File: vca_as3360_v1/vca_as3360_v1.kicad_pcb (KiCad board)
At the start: 2 copper layers, 30 x 100 mm, 71 parts, among them J1 Conn_02x05_Odd_Even, J2 OUT_1, J3 OUT_2, J4 CV1, J5 CV2, J6 IN1, J7 IN2, Q1 BC547, Q2 BC547, U1 AS3360, U2 TL072, U3 TL072, U4 TL072

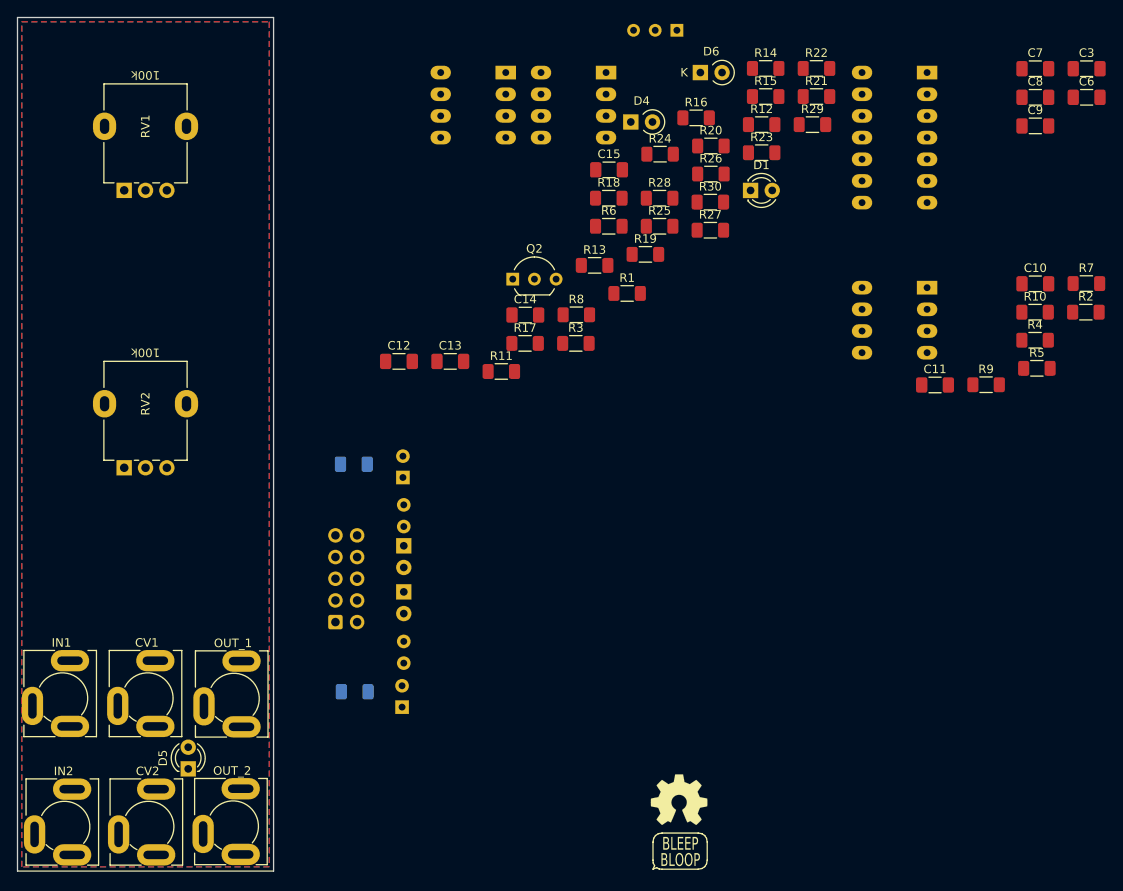
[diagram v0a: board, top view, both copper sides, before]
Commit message: Layout and routing first pass done
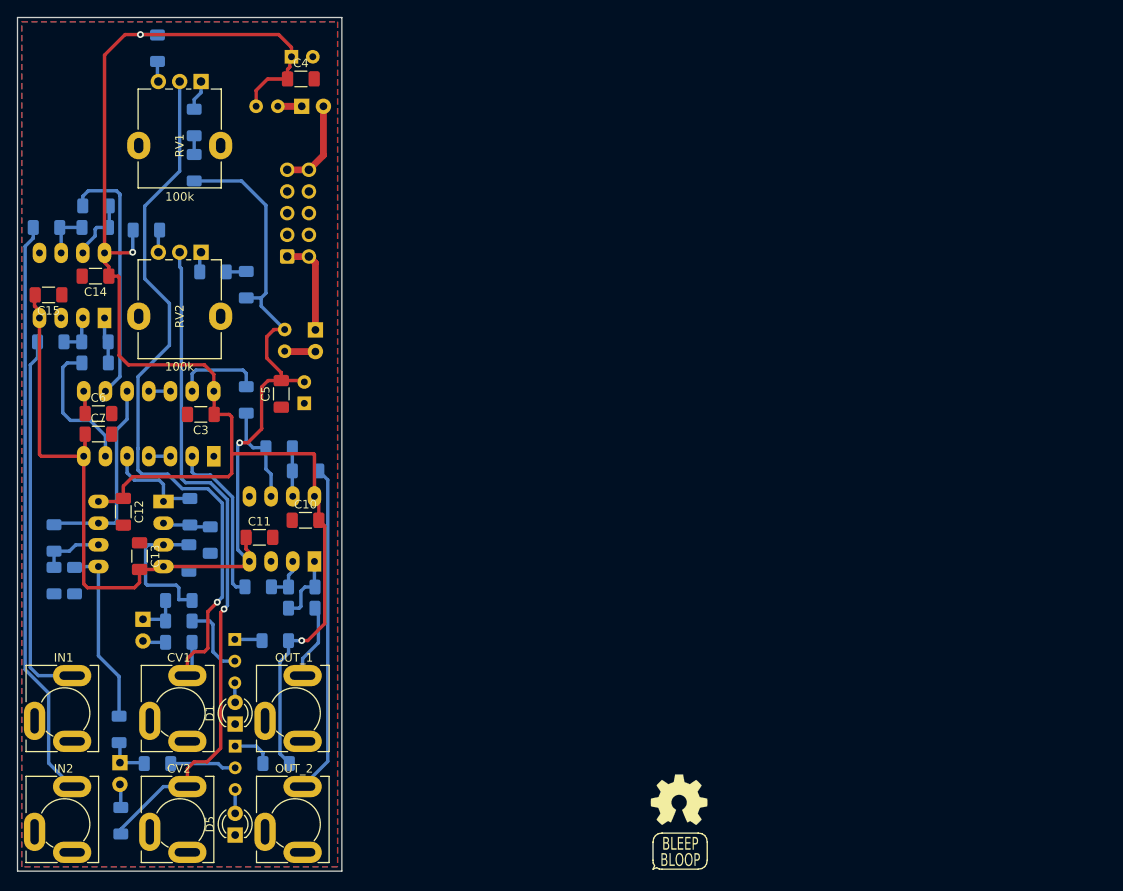
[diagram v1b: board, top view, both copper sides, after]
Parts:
- removed C8, C9: 10nF, Capacitor_SMD:C_1206_3216Metric_Pad1.33x1.80mm_HandSolder
- added R31: 10k, Resistor_SMD:R_1206_3216Metric_Pad1.30x1.75mm_HandSolder, B.Cu at (162.9, 79.8)
- added R32: 100k, Resistor_SMD:R_1206_3216Metric_Pad1.30x1.75mm_HandSolder, B.Cu at (166.8, 81.3)
- C4, C5: moved to F.Cu
- D4, D6, Q2, R1, R10, R12, R13, R14, R15, R17, R18, R19, R2, R21, R22, R23, R24, R26, R27, R28, R29, R3, R30, R4, R5, R6, R7, R8, R9: moved to B.Cu
- R11, R20: value R -> 1k; moved to B.Cu
- R16: value 90k -> 100k; moved to B.Cu
- R25: value 90k -> 10k; moved to B.Cu
- U3: value TL072 -> LM358
- moved C6 121.6 mm to (149.5, 96.4)
- moved R22 120.0 mm to (152.1, 144.1), turned to -90 degrees
- moved C7 117.8 mm to (149.5, 98.8)
- moved C3 111.4 mm to (161.5, 96.5), turned to 180 degrees
- moved R21 109.8 mm to (156.4, 137.4), turned to 180 degrees
- moved D6 105.6 mm to (152.0, 137.3), turned to -90 degrees
- moved R23 101.2 mm to (151.9, 133.4), turned to -90 degrees
- moved R2 98.2 mm to (173.3, 119.2), turned to 180 degrees
- moved R4 95.5 mm to (168.2, 116.7), turned to 180 degrees
- moved U1 94.9 mm to (163.0, 101.4), turned to 90 degrees
- moved R7 94.1 mm to (173.7, 103.1), turned to 180 degrees
- moved R14 92.8 mm to (158.9, 118.3), turned to 180 degrees
- moved R10 90.0 mm to (170.6, 100.4), turned to 180 degrees
- moved C10 89.9 mm to (173.7, 108.9)
- moved R5 89.9 mm to (173.3, 116.7), turned to 180 degrees
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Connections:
- R25 pad 1: -12V -> Net-(R16-Pad2)
- R25 pad 2: Net-(R25-Pad2) -> Net-(RV1-Pad1)
- RV1 pad 1: Net-(R16-Pad2) -> Net-(RV1-Pad1)
- RV2 pad 1: Net-(R25-Pad2) -> Net-(RV2-Pad1)
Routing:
- net +12V: track 0.00 -> 171.7 mm, vias 0 -> 3
- net -12V: track 0.00 -> 130.0 mm, vias 0 -> 1
- net Net-(J4-PadT): track 0.00 -> 88.2 mm, vias 0 -> 1
- net Net-(RV2-Pad2): track 0.00 -> 80.0 mm, vias 0 -> 1
- net Net-(J7-PadT): track 0.00 -> 68.2 mm
- net Net-(J6-PadT): track 0.00 -> 43.8 mm
- net Net-(J3-PadT): track 0.00 -> 38.6 mm
- net /intput_block/Signal_2: track 0.00 -> 29.7 mm
- net /intput_block/Linear CV 2: track 0.00 -> 23.3 mm
- net Net-(R23-Pad1): track 0.00 -> 21.4 mm
- net /output_block/OUT_A_BUF: track 0.00 -> 19.5 mm
- net Net-(R14-Pad1): track 0.00 -> 16.5 mm
- net /intput_block/Signal_1: track 0.00 -> 16.3 mm
- net /intput_block/Linear CV 1: track 0.00 -> 12.0 mm
- net Net-(R10-Pad2): track 0.00 -> 11.8 mm
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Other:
- board size 30 x 100 mm -> 38 x 100 mm
- board text added: "Could put connector here to pass power to another board making 4 x VCA"
- board text added: "HP Inch mm 1 0.2 5.08 2 0.4 10.16 3 0.6 15.24 4 0.8 20.32 5 1 25.4 6 1.2 30.48 7 1.4 35.56 8 1.6 40.64 9 1.8 45.72 10 2 50.8 11 2.2 55.88 12 2.4 60.96 13 2.6 66.04 14 2.8 71.12 15 3 76.2 16 3.2 81.28 17 3.4 86.36 18 3.6 91.44 19 3.8 96.52 20 4 101.6 21 4.2 106.68 22 4.4 111.76 23 4.6 116.84 24 4.8 121.92 25 5 127 26 5.2 132.08 27 5.4 137.16 28 5.6 142.24 29 5.8 147.32 30 6 152.4"
